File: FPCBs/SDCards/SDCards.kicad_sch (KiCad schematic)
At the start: 4 parts, among them J1 SD_Card_Device, J2 SD_Card_Device, J3 SD_Card_Device, J4 SD_Card_Device

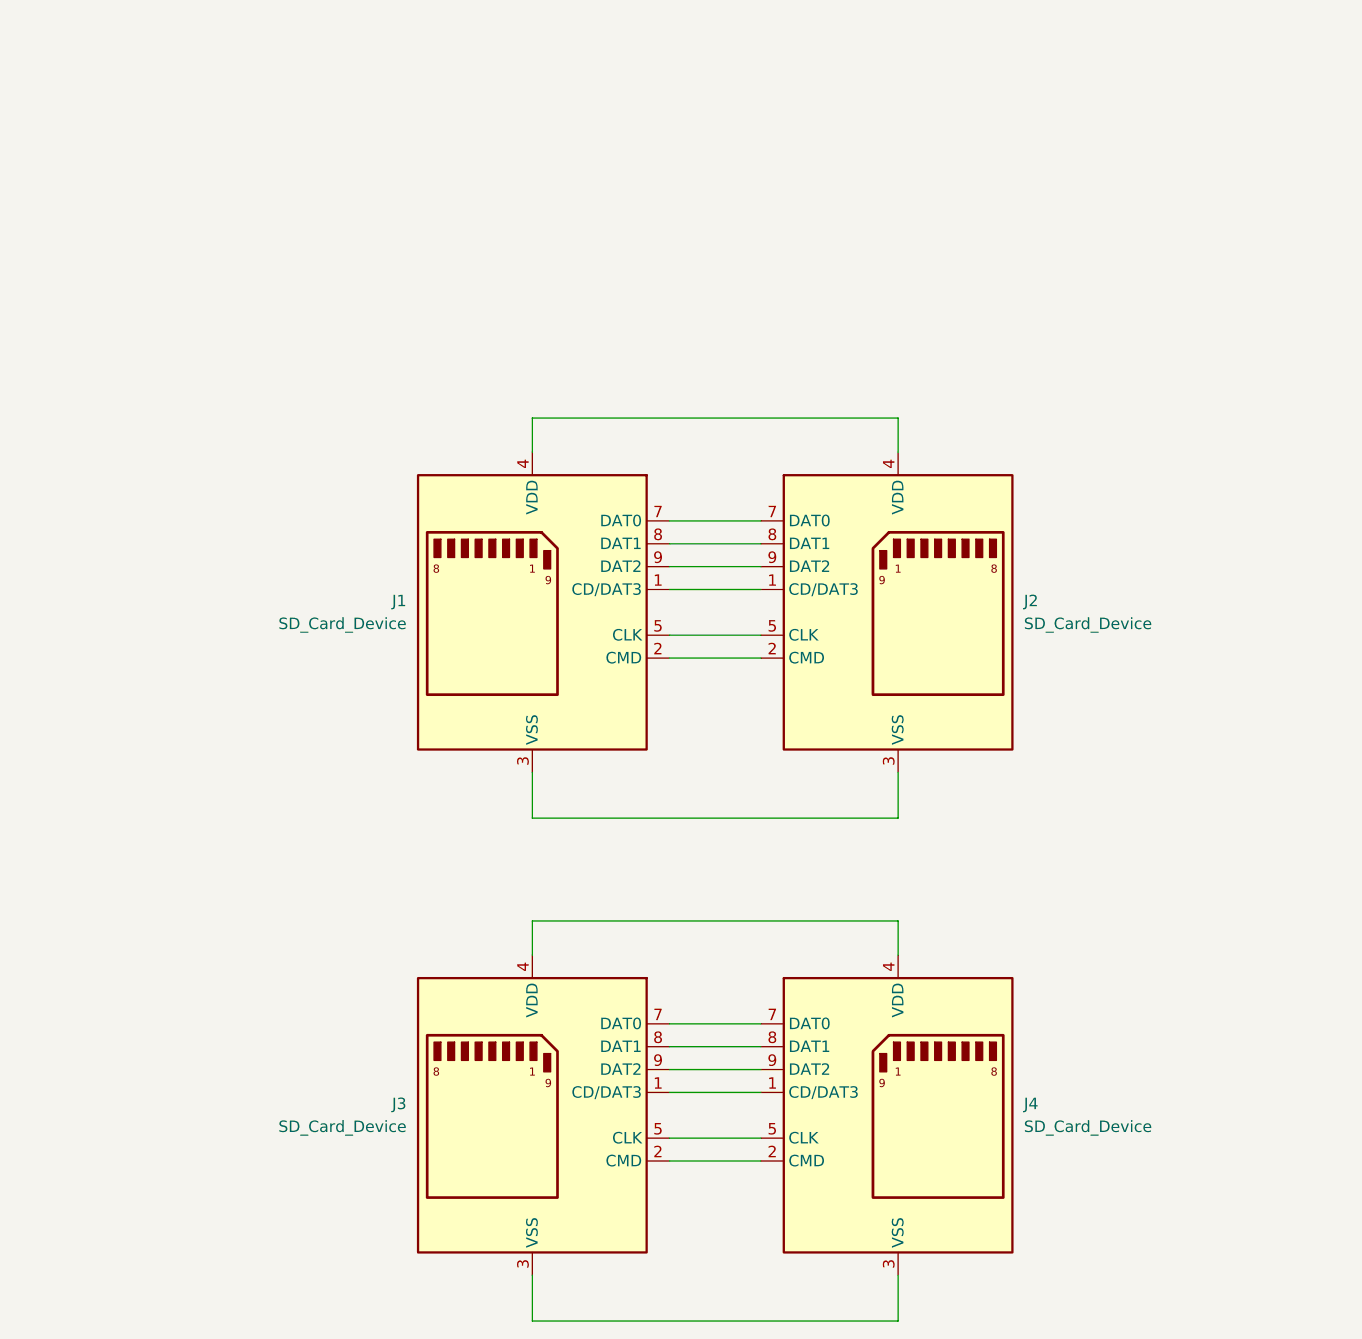
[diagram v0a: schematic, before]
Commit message: sd card
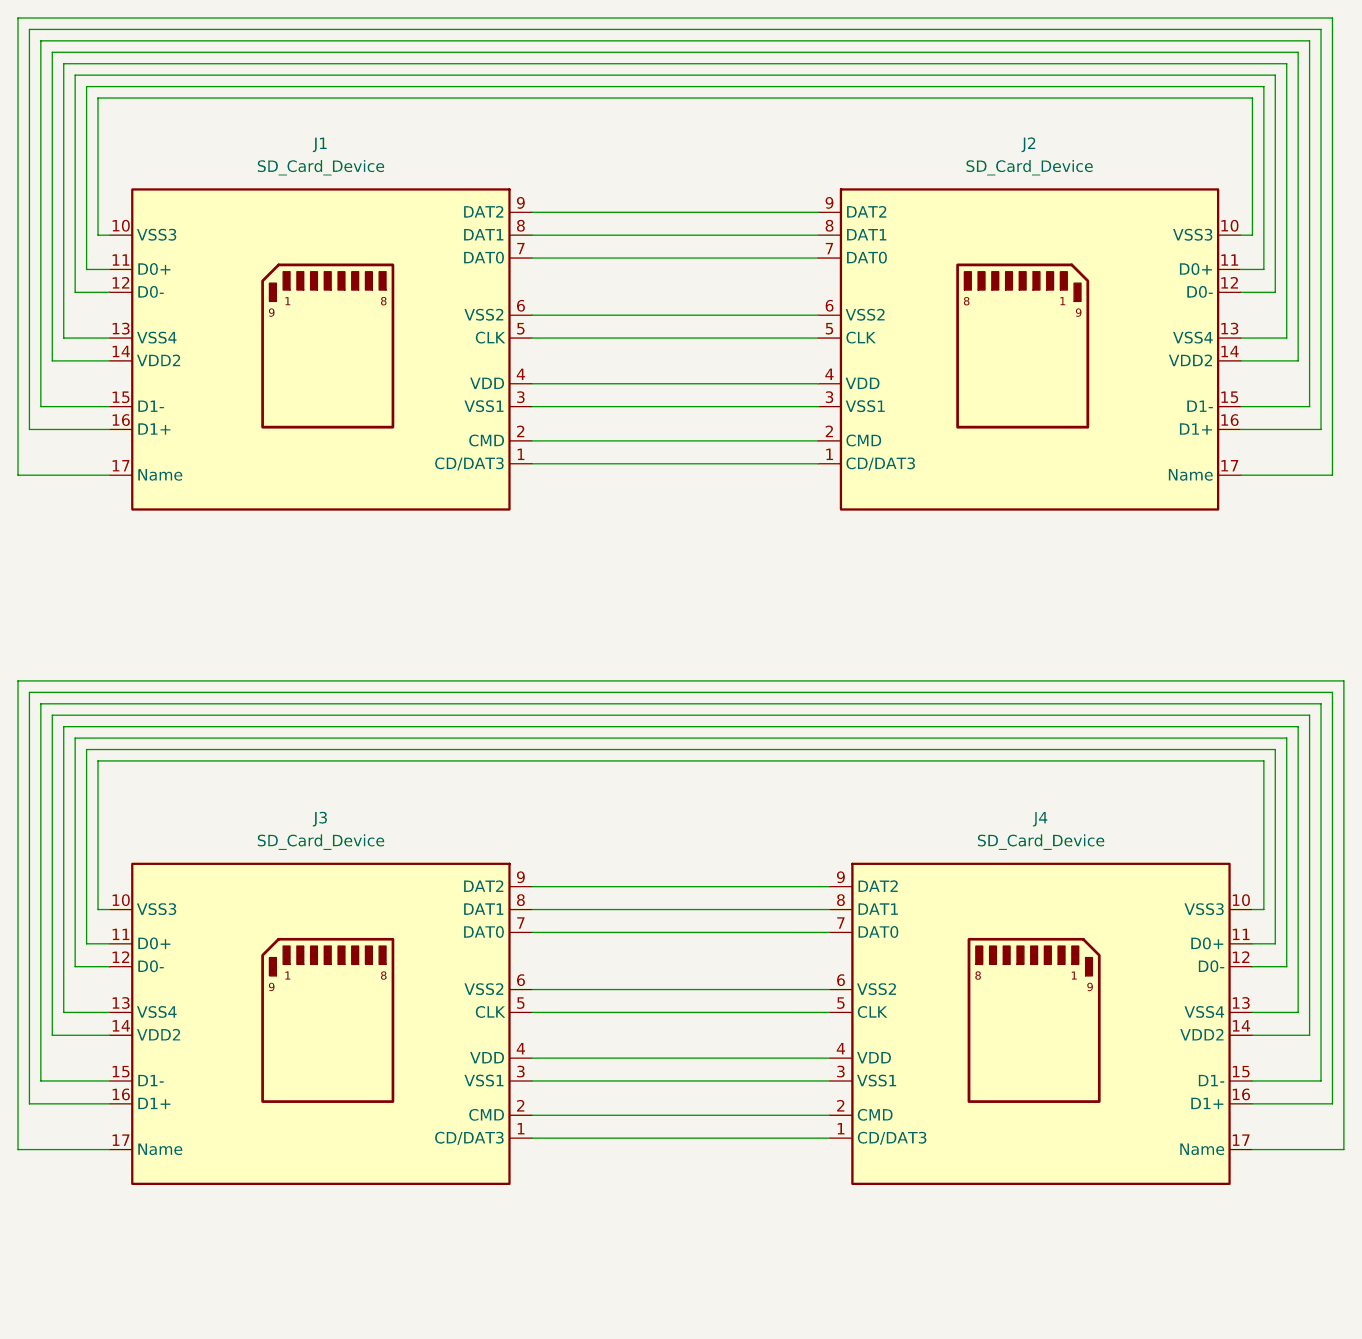
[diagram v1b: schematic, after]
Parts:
- J1, J2, J3, J4: symbol Connector:SD_Card_Device -> Leica-G9ii-Symbols:SD_Card_UHS2
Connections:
- net at J1.3 (VSS1), J2.3 (VSS1): no longer J1.6 (VSS), J2.6 (VSS)
- net at J3.3 (VSS1), J4.3 (VSS1): no longer J3.6 (VSS), J4.6 (VSS)
- new net: J1.10 (VSS3), J2.10 (VSS3)
- new net: J1.11 (D0+), J2.11 (D0+)
- new net: J1.12 (D0-), J2.12 (D0-)
- new net: J1.13 (VSS4), J2.13 (VSS4)
- new net: J1.14 (VDD2), J2.14 (VDD2)
- new net: J1.15 (D1-), J2.15 (D1-)
- new net: J1.16 (D1+), J2.16 (D1+)
- new net: J1.17 (Name), J2.17 (Name)
- new net: J1.6 (VSS2), J2.6 (VSS2)
- new net: J3.10 (VSS3), J4.10 (VSS3)
- new net: J3.11 (D0+), J4.11 (D0+)
- new net: J3.12 (D0-), J4.12 (D0-)
- new net: J3.13 (VSS4), J4.13 (VSS4)
- new net: J3.14 (VDD2), J4.14 (VDD2)
- new net: J3.15 (D1-), J4.15 (D1-)
- new net: J3.16 (D1+), J4.16 (D1+)
- new net: J3.17 (Name), J4.17 (Name)
- new net: J3.6 (VSS2), J4.6 (VSS2)
